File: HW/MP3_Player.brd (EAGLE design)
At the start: 210 x 15 mm, 75 parts, among them J2 LIPO-BATTERY-CONNECTOR, J3 USD-SDIO-SOCKETJLH, Q2 12.288MHz, U1 3.3V/150mA, U2 1.8V/100mA, U3 ATMEGA32U2, U4 VS1053B, U5 MCP73831

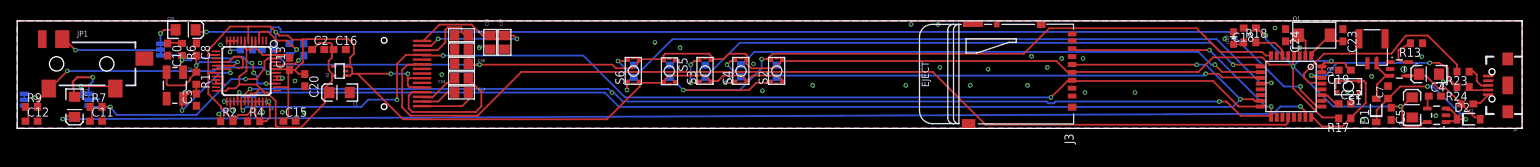
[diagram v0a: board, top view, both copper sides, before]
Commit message: Completed routing and verified. Added RC filters
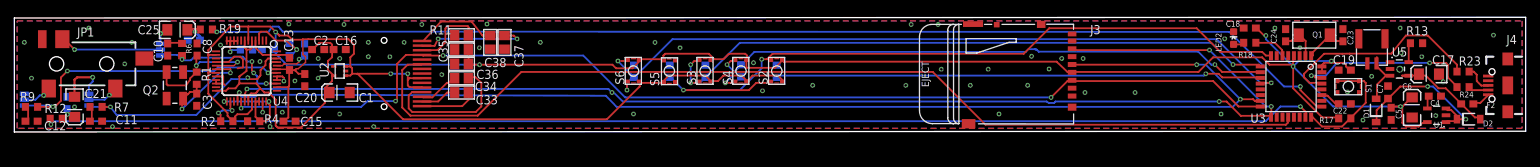
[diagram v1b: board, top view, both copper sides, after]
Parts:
- added C26, C27: 0.1uF, rcl:C0603
- added R12, R19: 68, rcl:R0603
- C21, C25: value (none) -> 10uF
- moved C25 1.15 mm to (22.4, 13.8)
- moved C8 0.10 mm to (25.1, 11.0)
- moved C9 0.10 mm to (40.1, 11.0)
- moved C3 0.05 mm to (25.1, 4.00)
- moved R1 0.05 mm to (25.1, 7.00)
- moved R18 0.05 mm to (172.0, 11.9)
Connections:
- net RCAP renamed N$33
- new net N$13: JP1.SLEEVE, JP4.2
- new net N$31: JP1.RING, JP3.2
- new net N$32: C21.A, C26.1, R12.1
- new net PWM_L1: C25.A, C27.1, R19.1
- net GBUF: no longer JP1.SLEEVE, JP4.2
- net GND: now also C26.2, C27.2
- net PWM_L: now also R12.2; no longer C21.A
- net PWM_R: now also R19.2; no longer C25.A
- net RIGHT: no longer JP1.RING, JP3.2
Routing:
- net RIGHT: track 35.2 -> 20.3 mm, vias 5 -> 4
- net N$31: track 0.00 -> 14.3 mm, vias 0 -> 1
- net N$14: track 11.5 -> 4.37 mm
- net N$13: track 0.00 -> 4.19 mm, vias 0 -> 1
- net GBUF: track 38.1 -> 42.1 mm
- net PWM_L1: track 0.00 -> 3.63 mm, vias 0 -> 1
- net N$32: track 0.00 -> 2.73 mm, vias 0 -> 1
- net PWM_R: track 162.9 -> 160.3 mm
- net N$4: track 4.74 -> 2.75 mm
- net N$28: track 3.74 -> 2.59 mm
- net PWM_L: track 177.0 -> 178.2 mm
- net N$46: track 19.6 -> 20.7 mm
- net N$48: track 9.64 -> 10.7 mm
- net N$55: track 11.1 -> 11.6 mm
- net GND: track 20.0 -> 19.8 mm, vias 37 -> 65
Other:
- board size 210 x 15 mm -> 210.9 x 16 mm
